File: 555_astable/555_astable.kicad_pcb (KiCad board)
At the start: 2 copper layers, 43 x 32.9 mm, 13 parts, among them J1 Conn_01x02, J2 Conn_01x03, SW1 SW_SPST, U1 NE555P

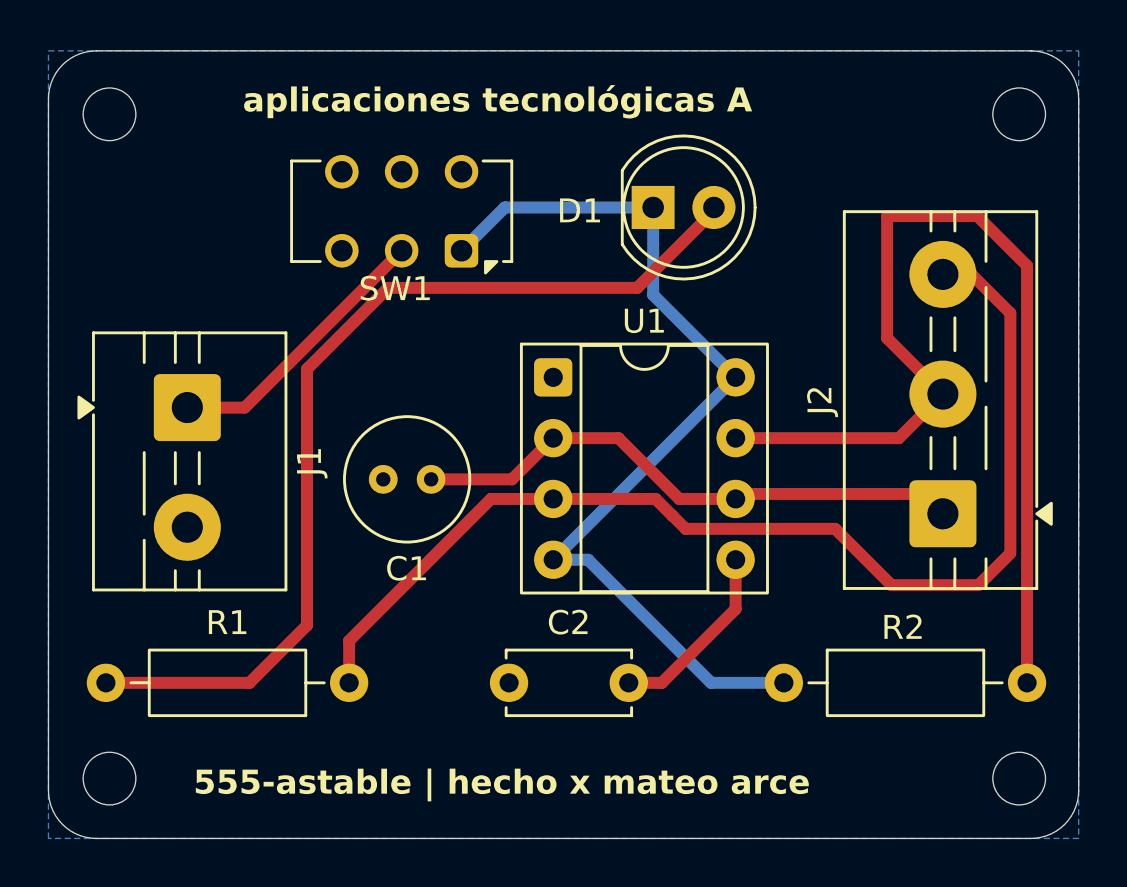
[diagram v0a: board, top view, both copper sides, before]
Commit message: actualizar 555 oficial
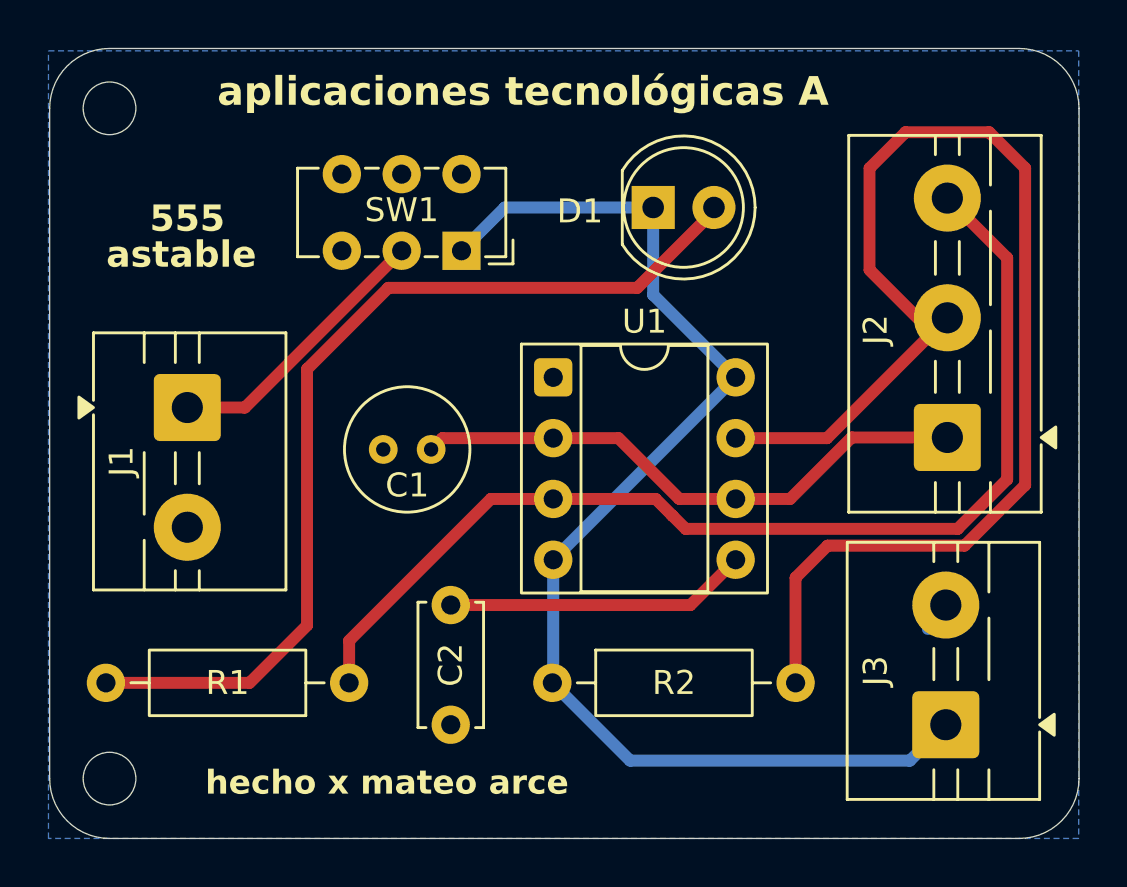
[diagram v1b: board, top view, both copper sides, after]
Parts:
- removed the REF** at (107.8, 38.8)
- removed the REF** at (107.8, 66.5)
- added J3: Conn_01x02, TerminalBlock:TerminalBlock_MaiXu_MX126-5.0-02P_1x02_P5.00mm, F.Cu at (104.7, 64.2)
- SW1: footprint Button_Switch_THT:SW_CK_JS202011CQN_DPDT_Straight -> Button_Switch_THT:SW_E-Switch_EG1271_SPDT
- moved R2 9.67 mm to (88.2, 62.5)
- moved J2 3.19 mm to (104.8, 52.2)
- moved C2 3.00 mm to (84.0, 64.2), turned to 90 degrees
- moved C1 1.25 mm to (83.2, 52.8)
- moved REF** 0.25 mm to (69.8, 38.5)
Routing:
- net Net-(J2-Pin_2): track 42.0 -> 55.8 mm
- net VCC: track 39.8 -> 51.6 mm
- net Net-(U1-CONT): track 7.80 -> 12.7 mm
- net Net-(J2-Pin_3): track 47.4 -> 45.9 mm
- net GND: track 0.00 -> 1.06 mm
- net Net-(J2-Pin_1): track 23.6 -> 24.2 mm
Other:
- board size 43 x 32.9 mm -> 43 x 33 mm
- board text added: "555"
- board text added: "astable"
- board text added: "hecho x mateo arce"
- board text removed: "555-astable | hecho x mateo arce"
